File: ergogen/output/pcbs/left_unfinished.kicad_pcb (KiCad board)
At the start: 2 copper layers, 140.9 x 102.2 mm, 49 parts

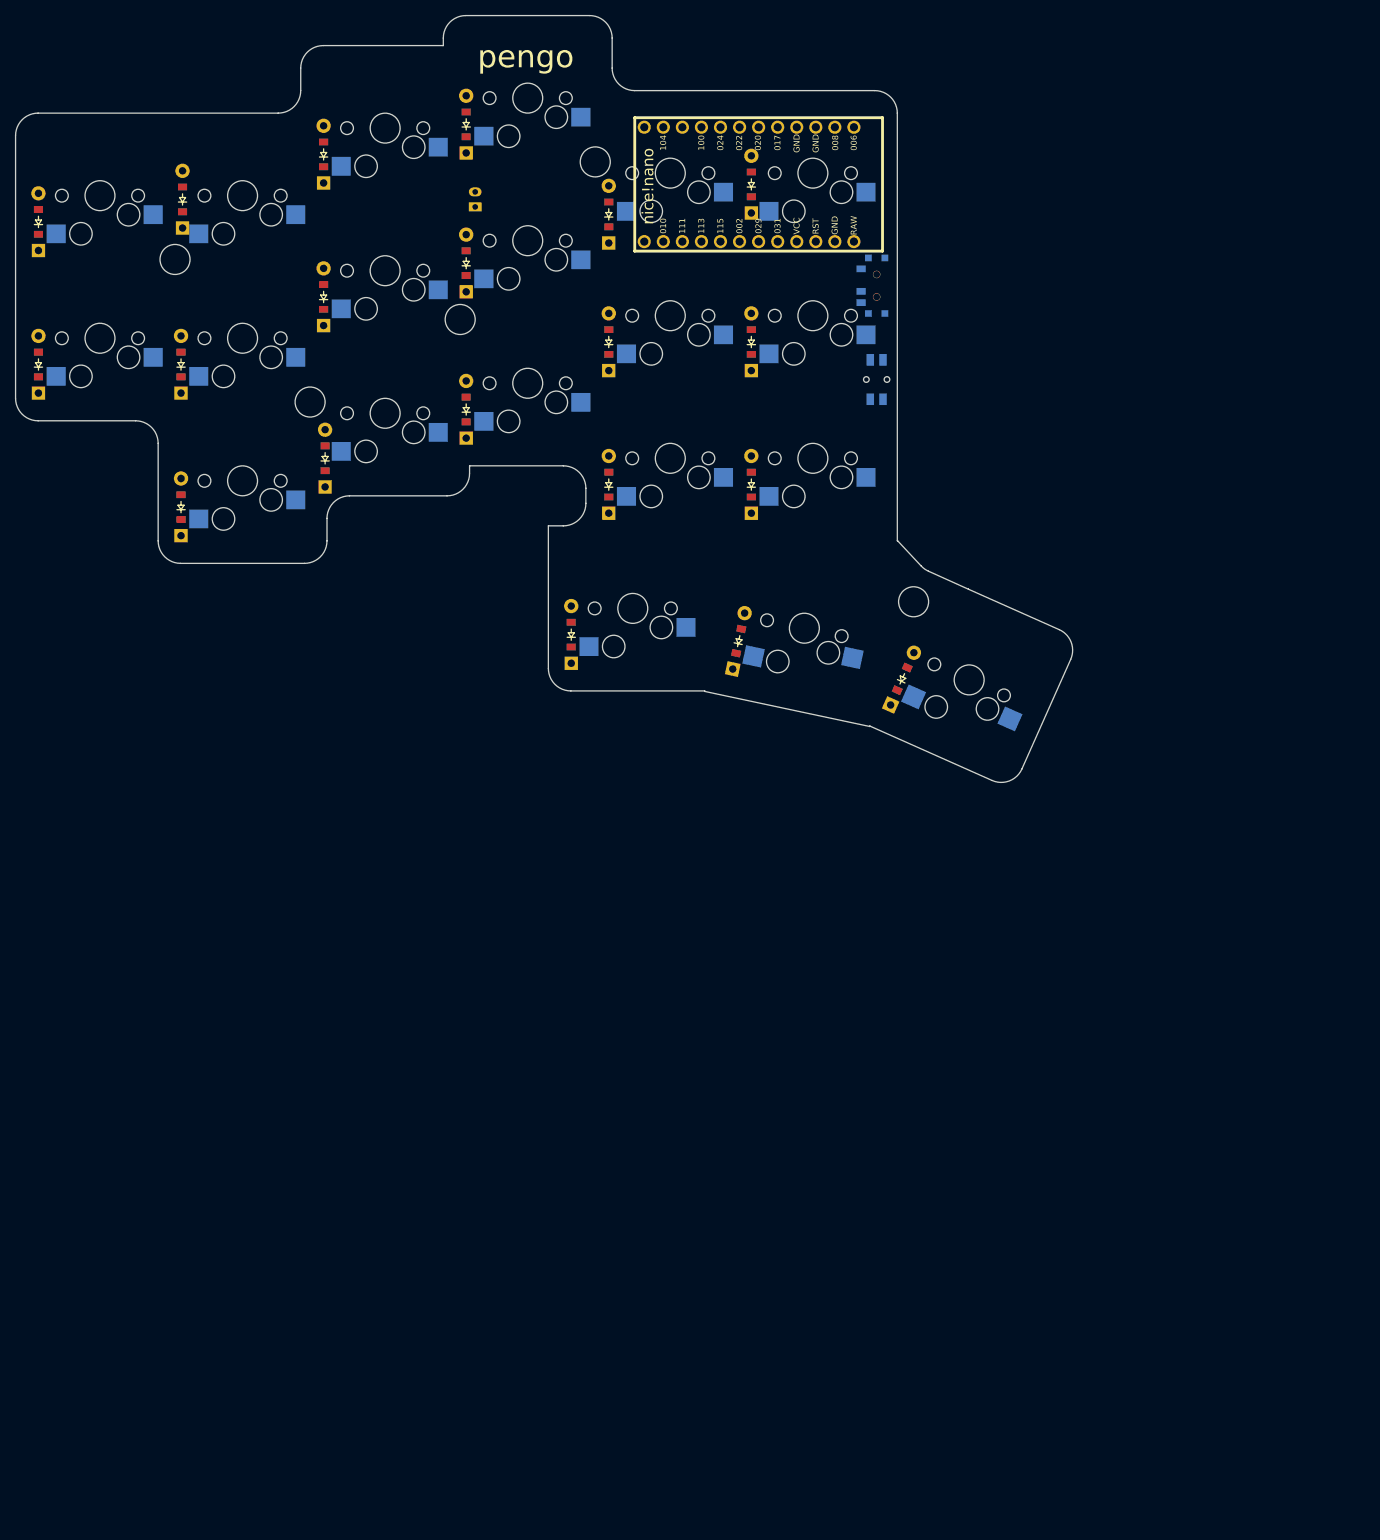
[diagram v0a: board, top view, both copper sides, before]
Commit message: Too many unrouted
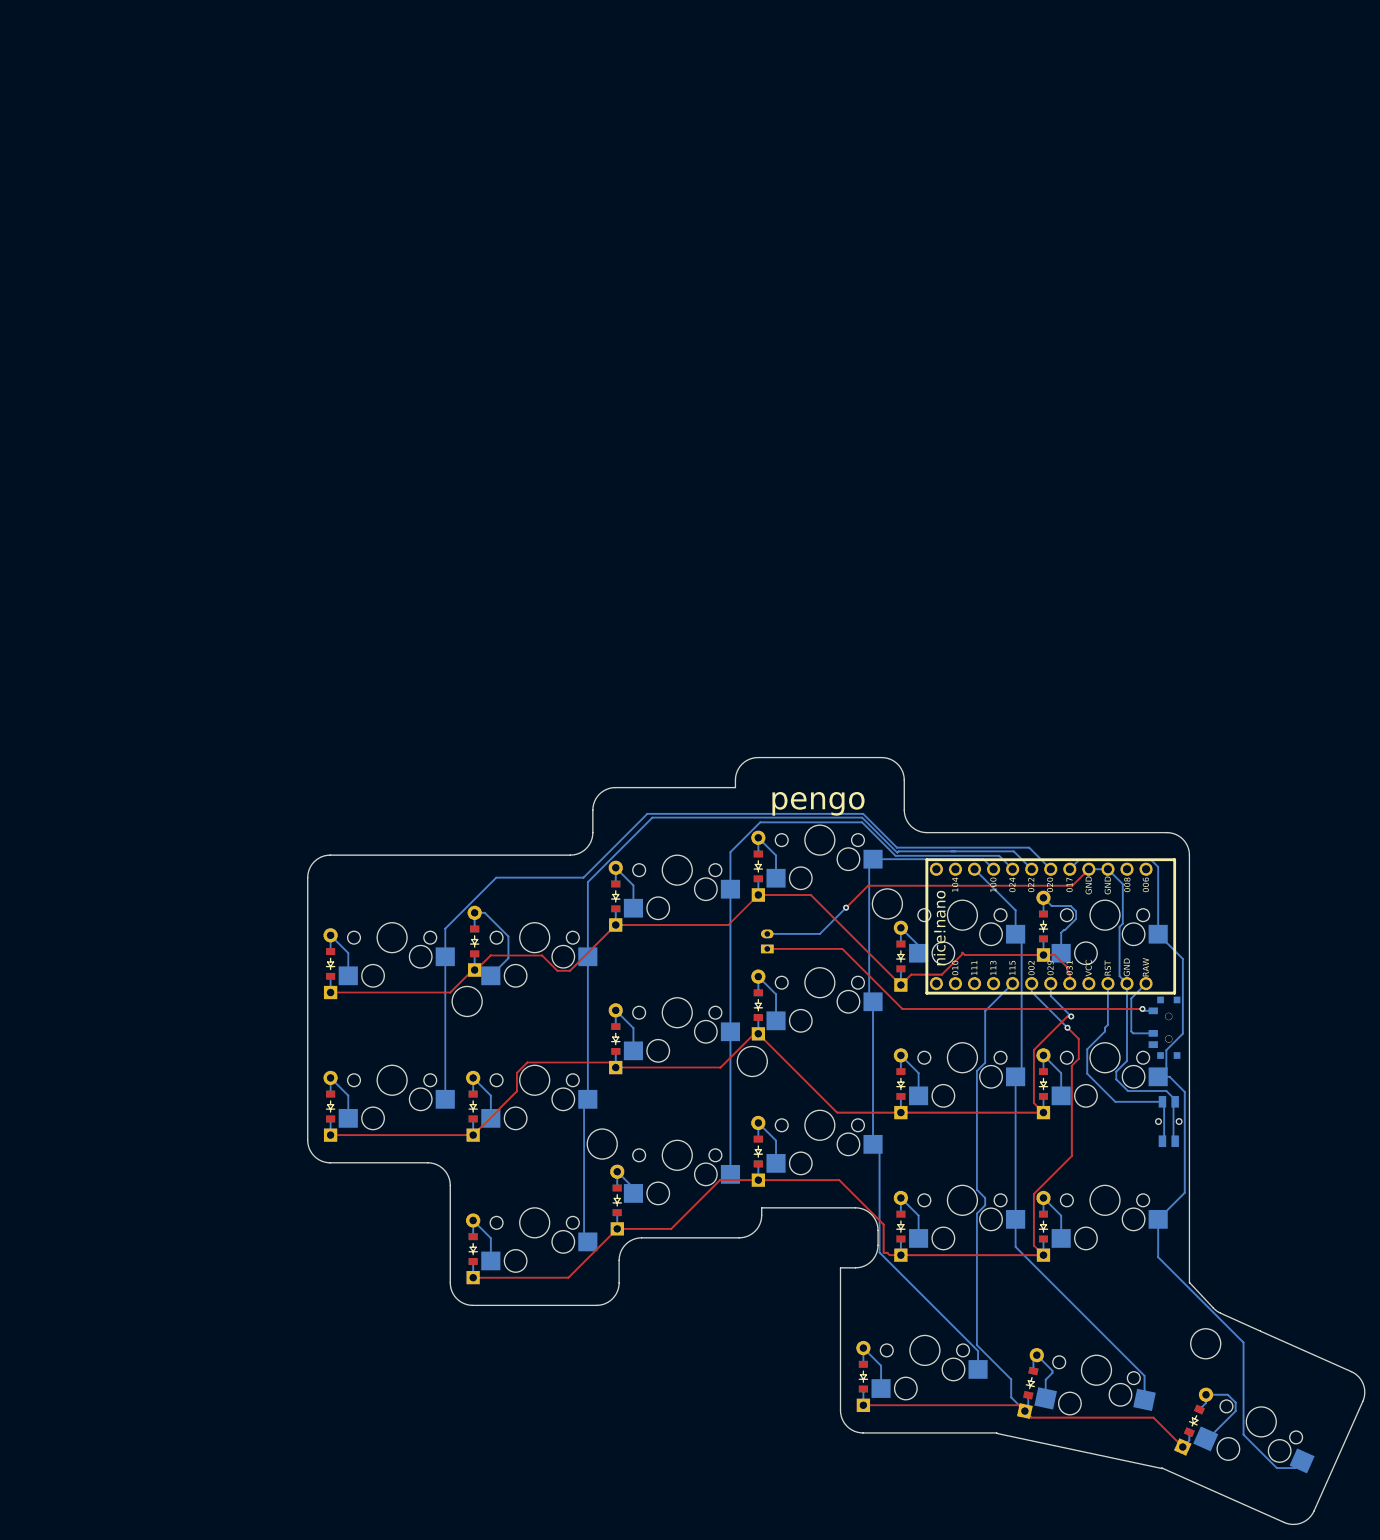
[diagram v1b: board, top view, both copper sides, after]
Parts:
- removed the ? at (108.4, 16.1)
- removed the ? at (28.0, -10.5)
- removed the ? at (10.0, -29.5)
- removed the ? at (66.0, -42.5)
- removed the ? at (48.0, -21.5)
- added ?: , HOLE_M2_TH, F.Cu at (48.9, 69.4)
- added ?: , HOLE_M2_TH, F.Cu at (104.9, 56.4)
- added ?: , HOLE_M2_TH, F.Cu at (66.9, 88.4)
- added ?: , HOLE_M2_TH, F.Cu at (147.4, 115.0)
- added ?: , HOLE_M2_TH, F.Cu at (86.9, 77.4)
- moved S20 106.3 mm to (154.8, 125.4)
- moved S19 106.3 mm to (132.8, 118.5)
- moved D14 106.3 mm to (124.0, 120.2)
- moved B1 106.3 mm to (142.4, 85.4)
- moved D1 106.3 mm to (30.7, 83.4)
- moved D10 106.3 mm to (106.7, 80.4)
- moved D11 106.3 mm to (125.7, 99.4)
- moved D12 106.3 mm to (125.7, 80.4)
- moved D13 106.3 mm to (101.7, 119.4)
- moved D16 106.3 mm to (49.9, 61.4)
- moved D17 106.3 mm to (68.9, 95.9)
- moved D18 106.3 mm to (87.7, 69.9)
- moved D19 106.3 mm to (106.7, 63.4)
- moved D2 106.3 mm to (30.7, 64.4)
- moved D20 106.3 mm to (125.7, 59.4)
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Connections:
- S1 pad 2: P029 -> outer_home
- S10 pad 2: P029 -> middle_home
- S11 pad 2: P031 -> middle_top
- S12 pad 2: P002 -> index_bottom
- S13 pad 2: P029 -> index_home
- S14 pad 2: P031 -> index_top
- S15 pad 2: P002 -> inner_bottom
- S16 pad 2: P029 -> inner_home
- S17 pad 2: P031 -> inner_top
- S18 pad 2: P115 -> near_thumb
- S19 pad 2: P115 -> home_thumb
- S2 pad 2: P031 -> outer_top
- S20 pad 2: P115 -> far_thumb
- S3 pad 2: P002 -> pinky_bottom
- S4 pad 2: P029 -> pinky_home
- S5 pad 2: P031 -> pinky_top
- S6 pad 2: P002 -> ring_bottom
- S7 pad 2: P029 -> ring_home
- S8 pad 2: P031 -> ring_top
- S9 pad 2: P002 -> middle_bottom
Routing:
- net P029: track 0.00 -> 141.1 mm, vias 0 -> 1
- net P002: track 0.00 -> 140.3 mm, vias 0 -> 1
- net P031: track 0.00 -> 128.2 mm
- net P022: track 0.00 -> 114.5 mm
- net P115: track 0.00 -> 114.2 mm
- net P020: track 0.00 -> 112.8 mm
- net P017: track 0.00 -> 109.6 mm
- net GND: track 0.00 -> 93.7 mm, vias 0 -> 1
- net P100: track 0.00 -> 90.8 mm
- net P024: track 0.00 -> 84.8 mm
- net P011: track 0.00 -> 80.8 mm
- net pos: track 0.00 -> 54.8 mm, vias 0 -> 1
- net RST: track 0.00 -> 30.2 mm
- net pinky_top: track 0.00 -> 14.2 mm
- net inner_top: track 0.00 -> 13.8 mm
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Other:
- net class Default removed

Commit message: done with the pcbs finally
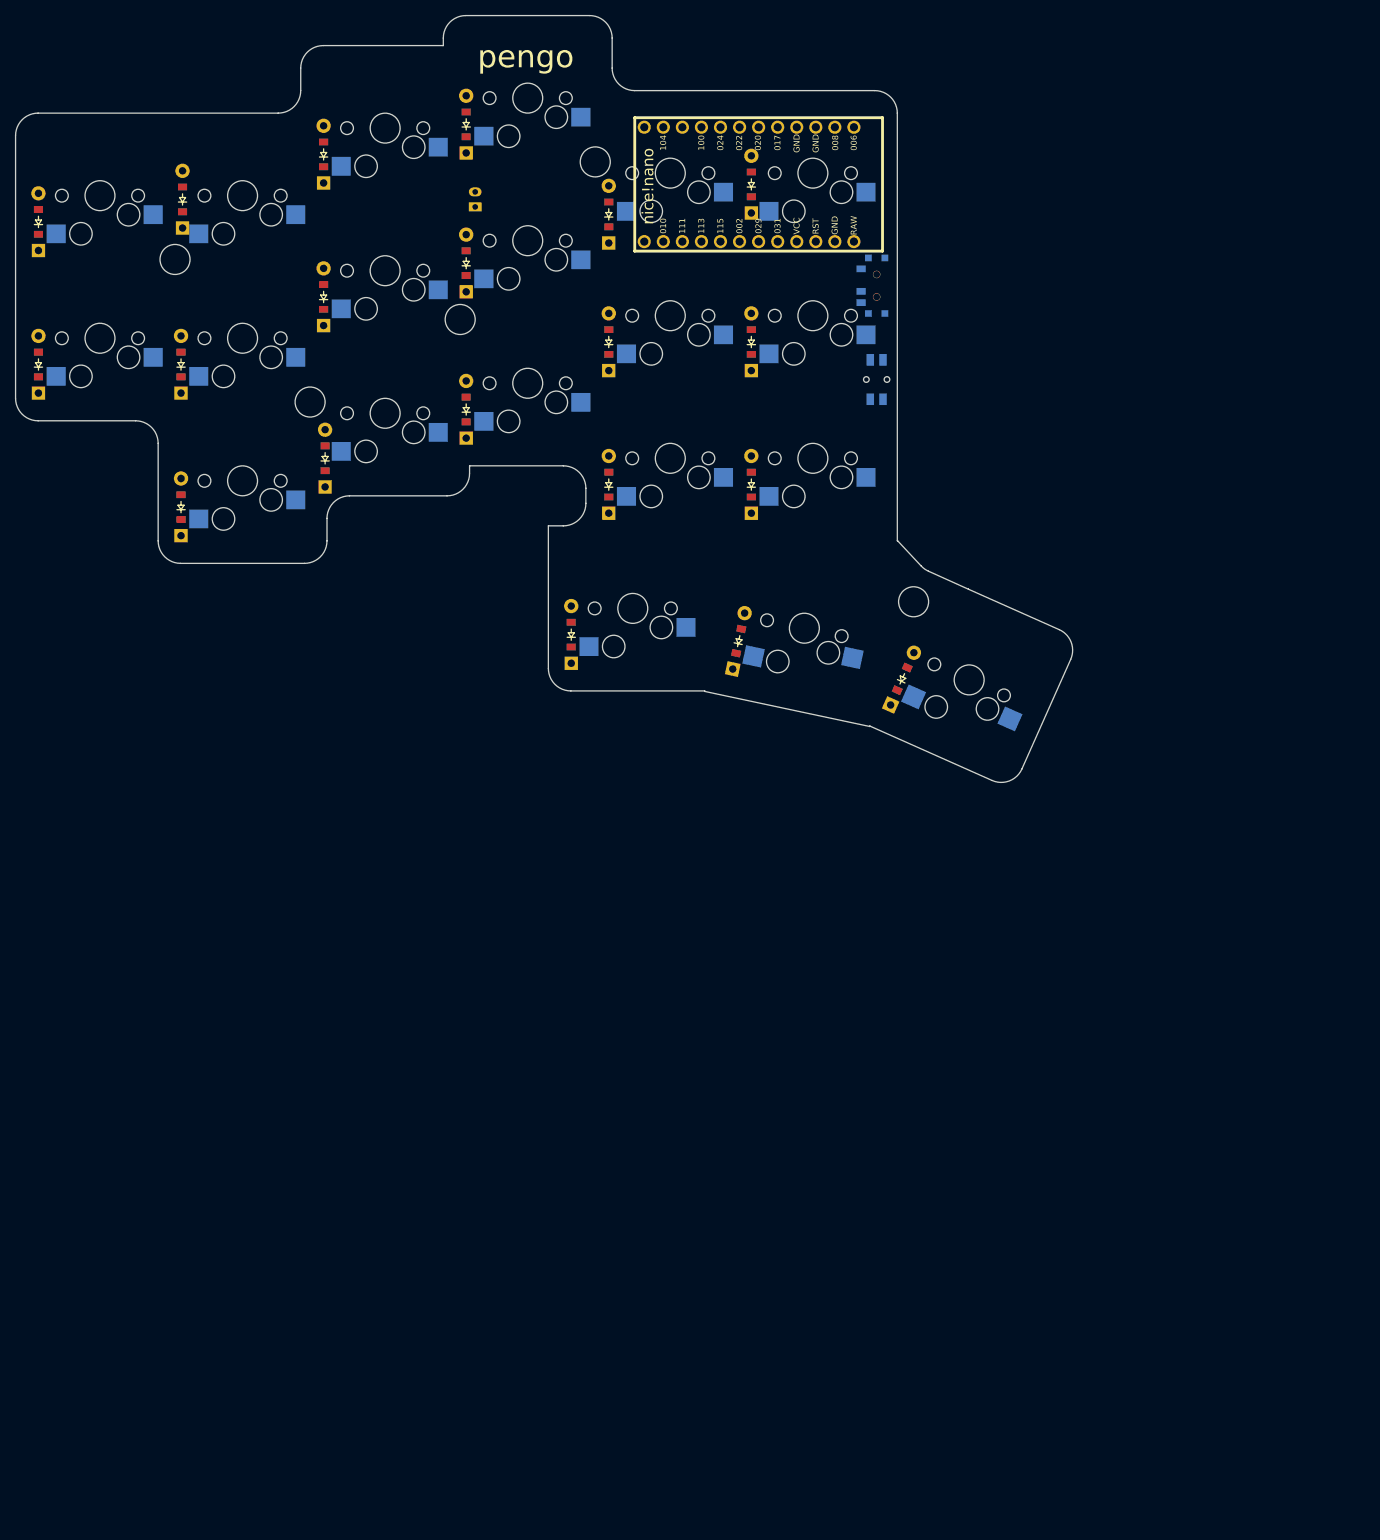
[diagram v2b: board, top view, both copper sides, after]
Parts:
- removed the ? at (48.9, 69.4)
- removed the ? at (104.9, 56.4)
- removed the ? at (66.9, 88.4)
- removed the ? at (147.4, 115.0)
- removed the ? at (86.9, 77.4)
- added ?: , HOLE_M2_TH, F.Cu at (108.4, 16.1)
- added ?: , HOLE_M2_TH, F.Cu at (28.0, -10.5)
- added ?: , HOLE_M2_TH, F.Cu at (10.0, -29.5)
- added ?: , HOLE_M2_TH, F.Cu at (66.0, -42.5)
- added ?: , HOLE_M2_TH, F.Cu at (48.0, -21.5)
- moved S20 106.3 mm to (115.8, 26.5)
- moved S19 106.3 mm to (93.9, 19.6)
- moved D14 106.3 mm to (85.1, 21.4)
- moved B1 106.3 mm to (103.5, -13.5)
- moved D1 106.3 mm to (-8.20, -15.5)
- moved D10 106.3 mm to (67.8, -18.5)
- moved D11 106.3 mm to (86.8, 0.50)
- moved D12 106.3 mm to (86.8, -18.5)
- moved D13 106.3 mm to (62.8, 20.5)
- moved D16 106.3 mm to (11.0, -37.5)
- moved D17 106.3 mm to (30.0, -3.00)
- moved D18 106.3 mm to (48.8, -29.0)
- moved D19 106.3 mm to (67.8, -35.5)
- moved D2 106.3 mm to (-8.20, -34.5)
- moved D20 106.3 mm to (86.8, -39.5)
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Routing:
- net P029: track 141.1 -> 0.00 mm, vias 1 -> 0
- net P002: track 140.3 -> 0.00 mm, vias 1 -> 0
- net P031: track 128.2 -> 0.00 mm
- net P022: track 114.5 -> 0.00 mm
- net P115: track 114.2 -> 0.00 mm
- net P020: track 112.8 -> 0.00 mm
- net P017: track 109.6 -> 0.00 mm
- net GND: track 93.7 -> 0.00 mm, vias 1 -> 0
- net P100: track 90.8 -> 0.00 mm
- net P024: track 84.8 -> 0.00 mm
- net P011: track 80.8 -> 0.00 mm
- net pos: track 54.8 -> 0.00 mm, vias 1 -> 0
- net RST: track 30.2 -> 0.00 mm
- net pinky_top: track 14.2 -> 0.00 mm
- net inner_top: track 13.8 -> 0.00 mm
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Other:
- net class Default added: clearance 0.2, trace_width 0.25, via_dia 0.8, via_drill 0.4
